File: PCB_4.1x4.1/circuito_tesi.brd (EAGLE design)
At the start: 100 x 80 mm, 43 parts, among them IC1 SCD41-D-R2, IC2 TPS60120PWPR, IC3 TPS78918DBVR, Q1 BSS138, Q2 BSS138, Q3 BSS138, Q4 BSS138, U1 TSV912IDT, U2 SGP30, U3 MICS-6814, U5 317030213, U6 BME280, U7 LIS3DH, U8 MAX682ESA+

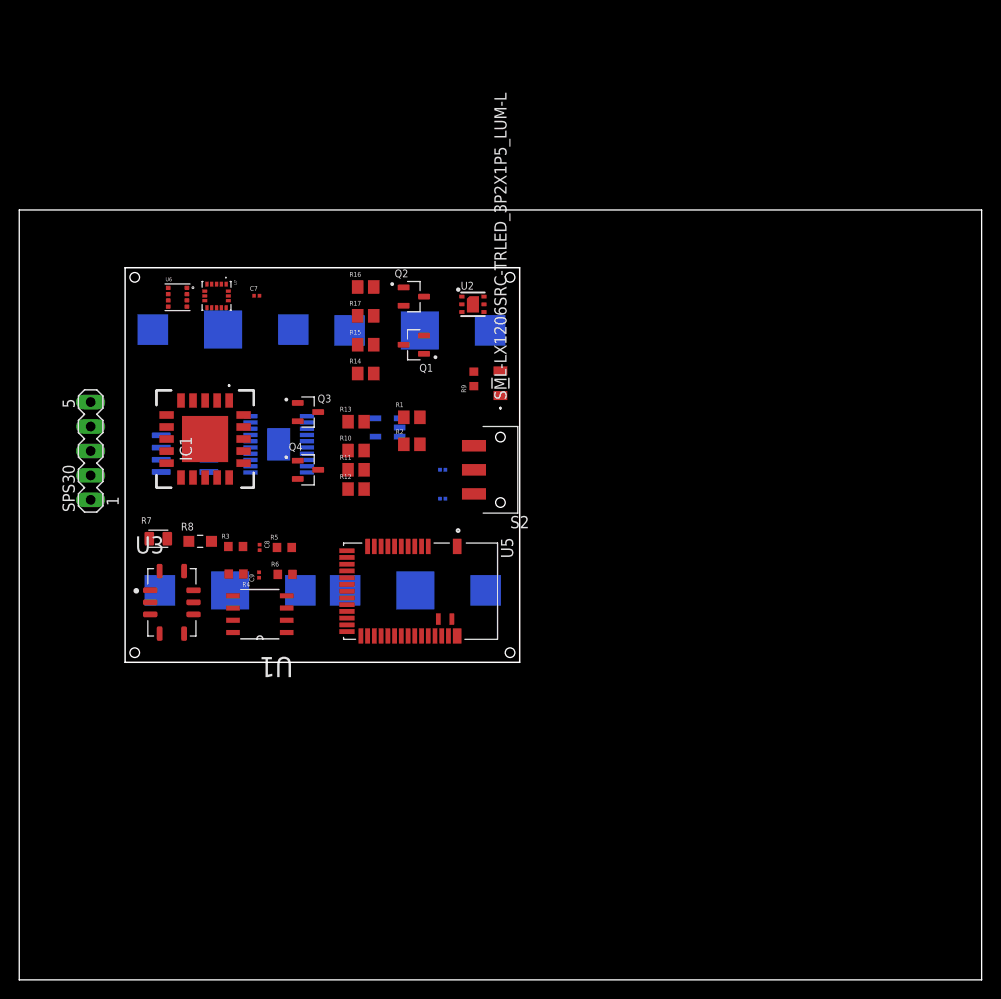
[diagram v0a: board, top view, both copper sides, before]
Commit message: PCB prima prova
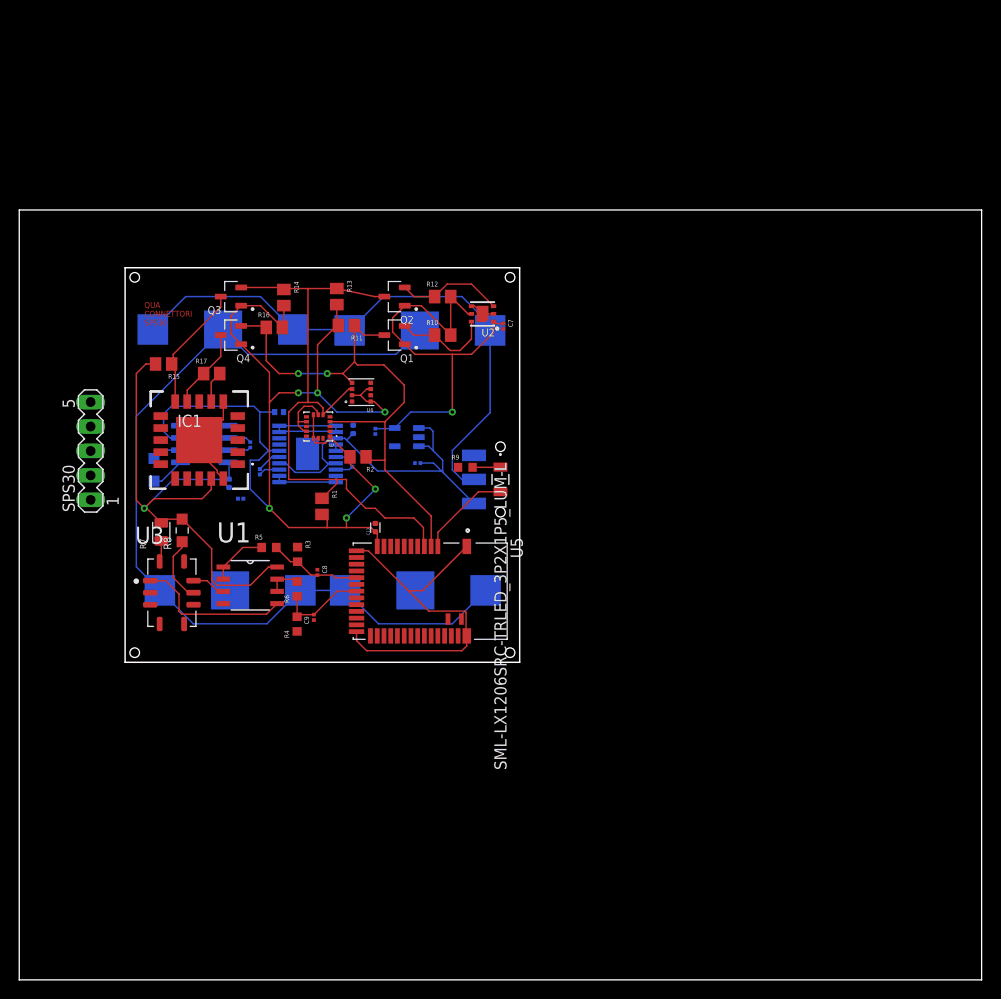
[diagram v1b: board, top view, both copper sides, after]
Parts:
- added C1, C12, C13: CL05A106MP5NUNC, Condens_10uF:CAPC1005X55N
- added C2, C3, C5: GRM033R61A225KE47D, Condens_2.2uF:CAPC0603X39N
- added C4: CL05A226MQ5N6J8, Condens_22uF:CAPC1005X55N
- added C6: GRM033R60J105MEA2D, Condens_1uF:CAPC0603X35N
- added R18: ERA6VEB8200V, Res_820_0p25W:RES_ERA6VEB8200V
- moved C7 25.8 mm to (50.3, 67.9), turned to 270 degrees
- moved R12 21.9 mm to (44.0, 71.0)
- moved U6 21.5 mm to (35.5, 61.1), turned to 180 degrees
- moved R15 21.1 mm to (15.0, 64.0), turned to 180 degrees
- moved U7 17.2 mm to (31.1, 57.5), turned to 180 degrees
- moved R17 17.1 mm to (20.0, 63.0)
- moved Q4 16.1 mm to (22.0, 67.0), turned to 180 degrees
- moved R11 15.0 mm to (34.0, 68.0), turned to 180 degrees
- moved R10 15.0 mm to (44.0, 67.0)
- moved Q3 14.4 mm to (22.0, 71.0), turned to 180 degrees
- moved R13 13.2 mm to (33.0, 71.0), turned to 270 degrees
- moved R1 13.2 mm to (31.5, 49.2), turned to 270 degrees
- moved R14 11.6 mm to (27.5, 70.9), turned to 270 degrees
- moved R16 10.4 mm to (26.5, 67.8)
- moved LED2 10.0 mm to (50.0, 52.0), turned to 270 degrees
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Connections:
- new net N$12: C2.1, IC2.8
- new net N$14: C3.2, IC2.15
- new net N$18: C3.1, IC2.13
- new net N$19: IC2.4, IC2.5
- new net N$20: C6.2, U8.6
- new net N$22: C6.1, U8.7
- new net N$24: R18.1, U8.2
- new net N$7: C2.2, IC2.6
- net 3.3: now also C13.1, C4.2, C5.2, Q4.1, R16.2, R18.2; no longer IC1.19, IC1.7
- net 5V: now also C12.1, IC1.19, IC1.7; no longer Q4.1, R16.2
- net GND: now also C1.2, C12.2, C13.2, C4.1, C5.1
- net N$1: now also IC1.10
- net N$15: now also U5.18; no longer U5.16
- net N$17: now also U5.16; no longer U5.18
- net N$21: now also U5.2; no longer U5.27
- net N$3: now also IC1.9
- net SCL: now also U5.3; no longer IC1.9, U5.26
- net SDA: now also U5.4; no longer IC1.10, U5.25
- net VDD: now also C1.1
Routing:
- net 3.3: track 0.00 -> 131.5 mm, vias 0 -> 6
- net N$4: track 0.00 -> 94.0 mm
- net GND: track 0.00 -> 77.9 mm
- net SDA: track 0.00 -> 64.2 mm
- net 5V: track 0.00 -> 60.9 mm, vias 0 -> 1
- net N$2: track 0.00 -> 60.0 mm
- net SCL: track 0.00 -> 58.6 mm, vias 0 -> 2
- net 1.8V: track 0.00 -> 45.5 mm, vias 0 -> 1
- net VDD: track 0.00 -> 40.0 mm
- net N$6: track 0.00 -> 16.1 mm
- net N$1: track 0.00 -> 13.2 mm
- net N$16: track 0.00 -> 11.1 mm
- net N$23: track 0.00 -> 10.3 mm
- net N$21: track 0.00 -> 9.71 mm
- net N$17: track 0.00 -> 9.64 mm
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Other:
- board text added: "QUA CONNETTORI SPS30"
